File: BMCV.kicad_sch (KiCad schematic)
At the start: 32 parts, among them J13 DebugPins, J14 USB_C_Receptacle_USB2.0_14P, SW14 Reset, SW15 Boot, U32 TXS0108EPW, U36 STM32G474CETx, U37 MB85RS64PNF-G-JNERE1, Y1 38.4MHz 10pF

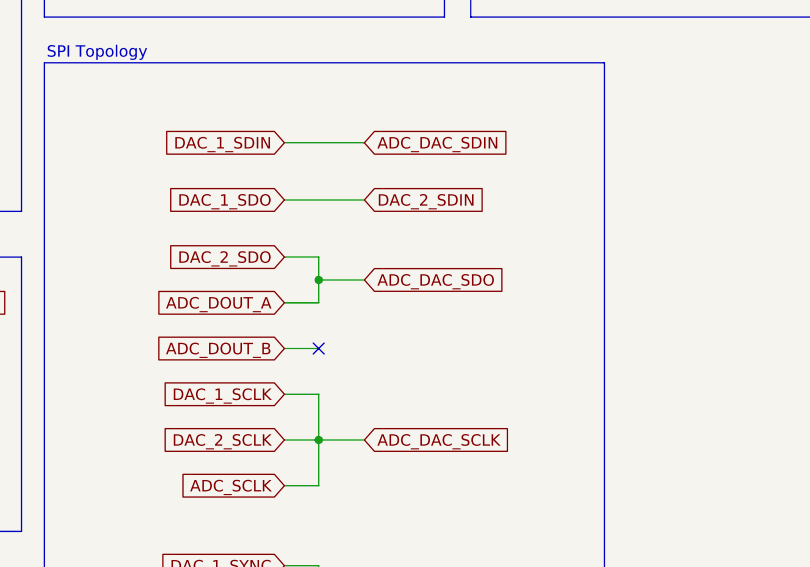
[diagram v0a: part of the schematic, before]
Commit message: pcb changes
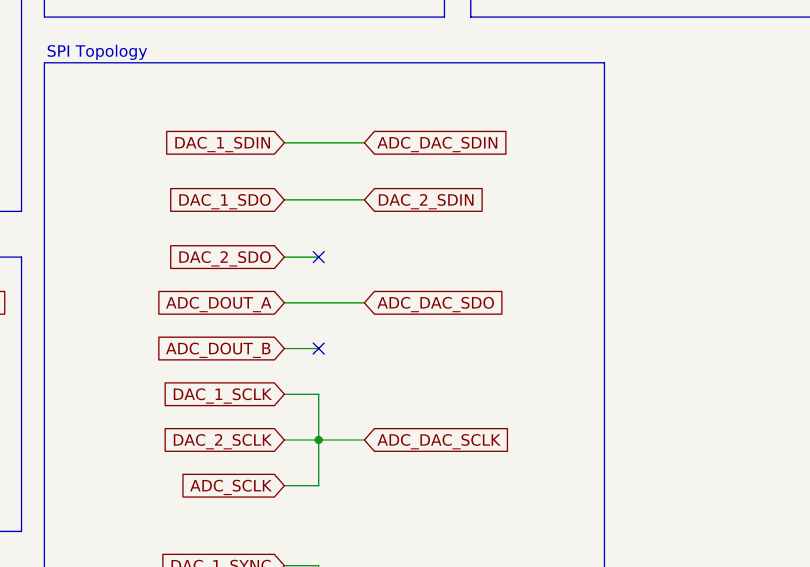
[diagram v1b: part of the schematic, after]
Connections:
- no-connect marks 3 -> 4
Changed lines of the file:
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@@
 	)
 	(junction
-		(at 140.97 175.26)
-		(diameter 0)
-		(color 0 0 0 0)
-	)
-	(junction
 		(at 29.21 237.49)
 		(diameter 0)
@@
 	)
 	(no_connect
+		(at 140.97 172.72)
+	)
+	(no_connect
 		(at 64.77 114.3)
 	)
@@
 	(wire
 		(pts
-			(xy 140.97 177.8) (xy 137.16 177.8)
+			(xy 137.16 177.8) (xy 146.05 177.8)
 		)
 		(stroke
@@
 	(wire
 		(pts
-			(xy 140.97 172.72) (xy 140.97 175.26)
-		)
-		(stroke
-			(width 0)
-			(type default)
-		)
-	)
-	(wire
-		(pts
 			(xy 118.11 269.24) (xy 128.27 269.24)
 		)
@@
 	(wire
 		(pts
-			(xy 140.97 175.26) (xy 146.05 175.26)
-		)
-		(stroke
-			(width 0)
-			(type default)
-		)
-	)
-	(wire
-		(pts
 			(xy 20.32 157.48) (xy 20.32 146.05)
 		)
@@
 	(wire
 		(pts
-			(xy 140.97 175.26) (xy 140.97 177.8)
-		)
-		(stroke
-			(width 0)
-			(type default)
-		)
-	)
-	(wire
-		(pts
 			(xy 69.85 257.81) (xy 72.39 257.81)
 		)
@@
 	(global_label "ADC_DAC_SDO"
 		(shape input)
-		(at 146.05 175.26 0)
+		(at 146.05 177.8 0)
 		(fields_autoplaced yes)
 		(effects
@@
 		)
 		(property "Intersheetrefs" "${INTERSHEET_REFS}"
-			(at 162.0376 175.26 0)
+			(at 162.0376 177.8 0)
 			(effects
 				(font

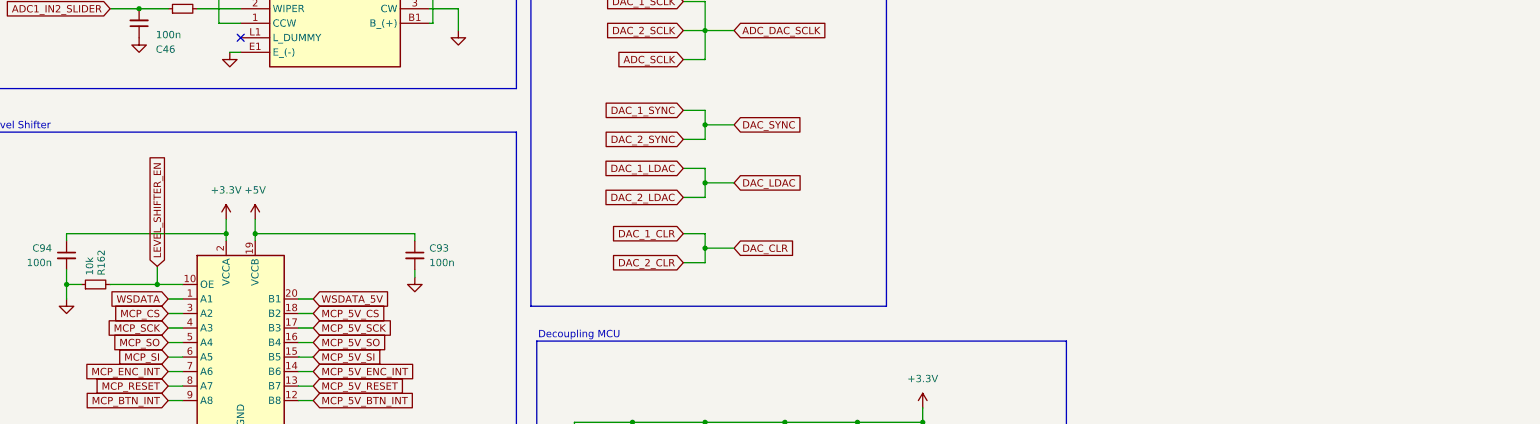
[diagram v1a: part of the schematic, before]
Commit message: pcb
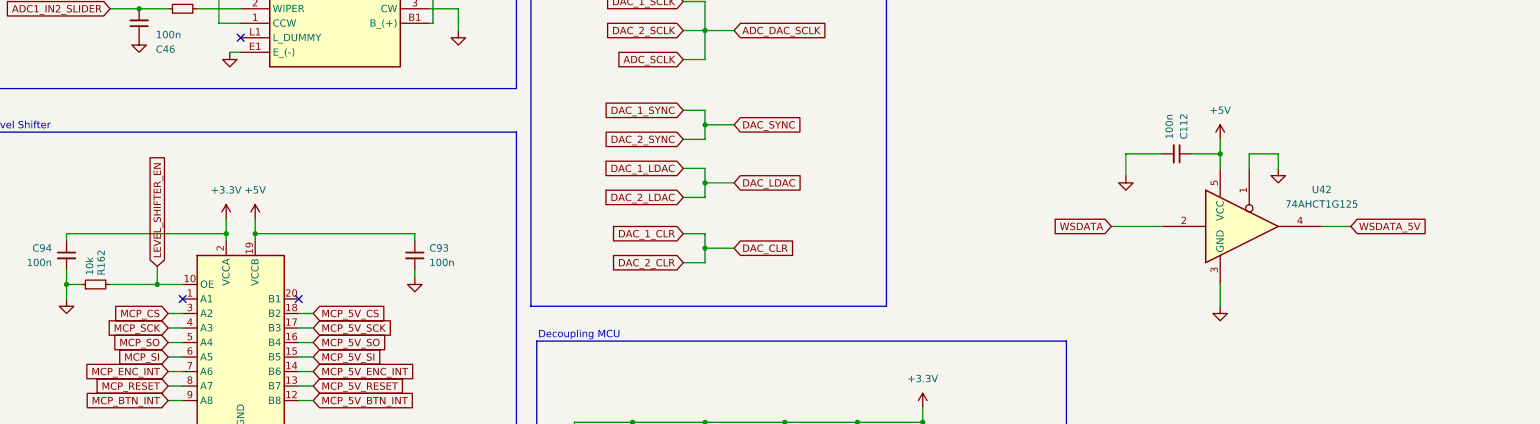
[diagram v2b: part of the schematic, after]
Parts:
- added C112: 100n, Capacitor_SMD:C_0402_1005Metric, symbol Device:C_Small
- added U42: 74AHCT1G125, Package_TO_SOT_SMD:SOT-353_SC-70-5, symbol 74xGxx:74AHCT1G125
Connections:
- net +5V: now also C112.1, U42.5 (VCC)
- net GND: now also C112.2, U42.1, U42.3 (GND)
- net WSDATA: now also U42.2; no longer U32.1 (A1)
- net WSDATA_5V: now also U42.4; no longer U32.20 (B1)
- no-connect marks 4 -> 6

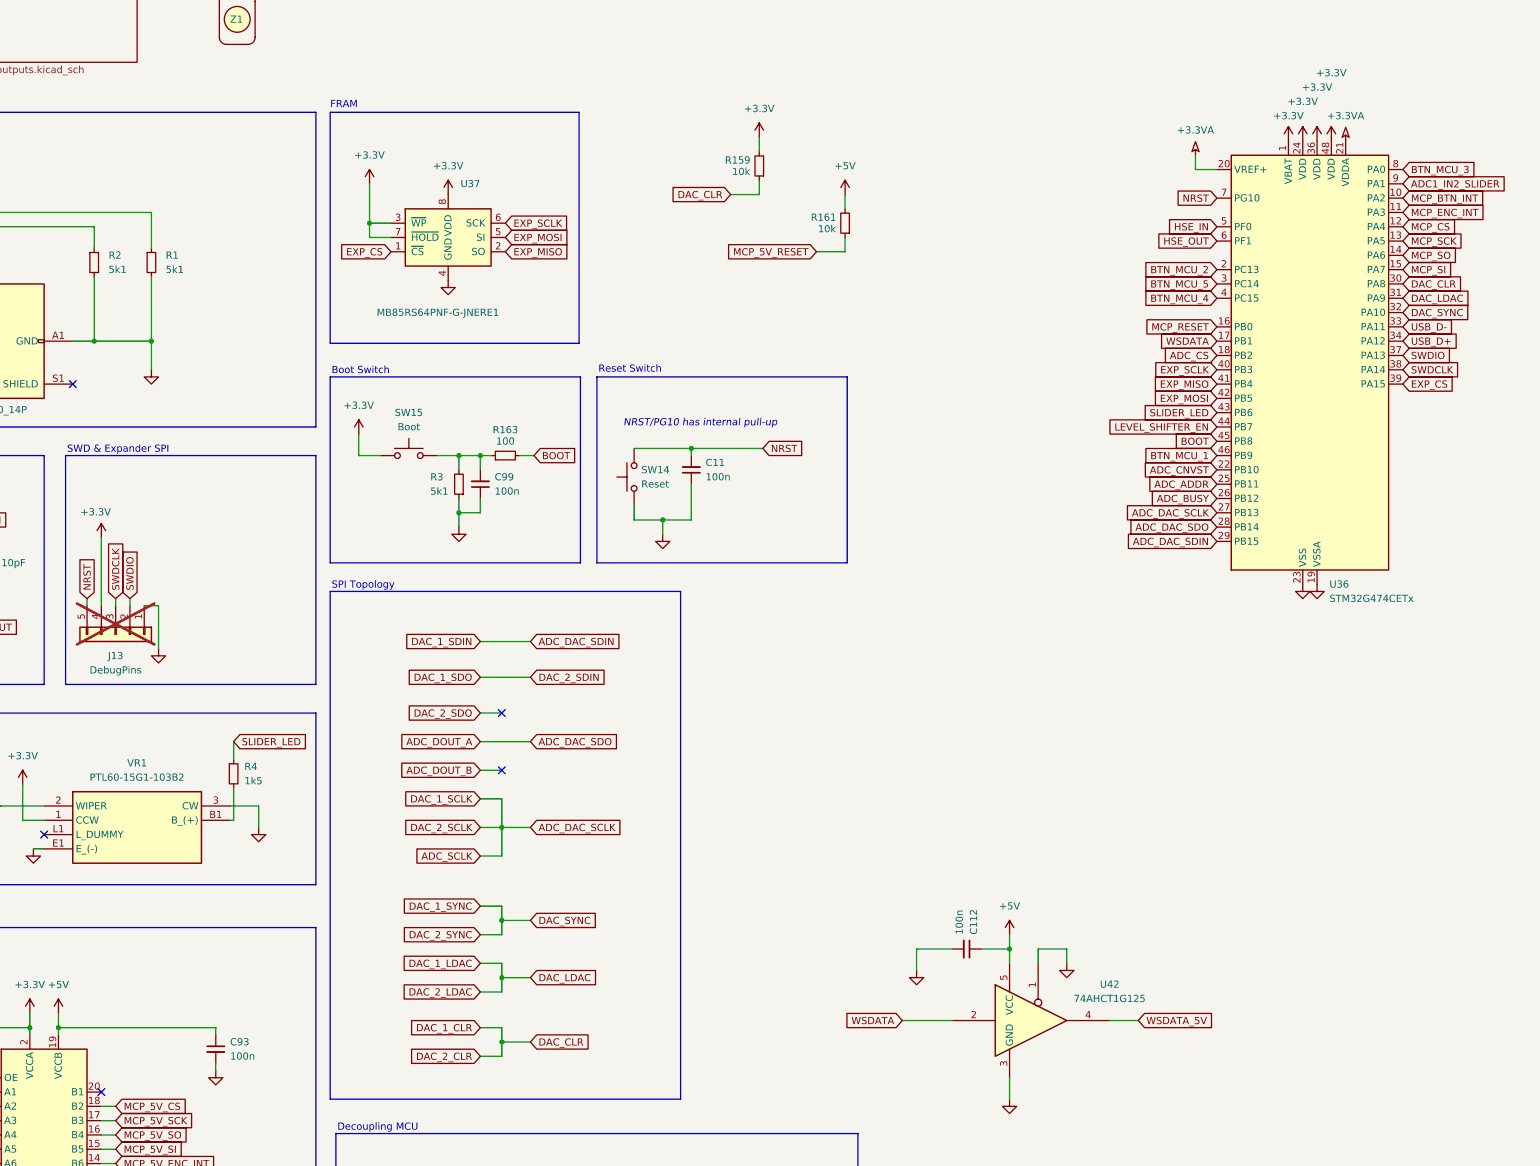
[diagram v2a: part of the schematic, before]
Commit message: pcb update
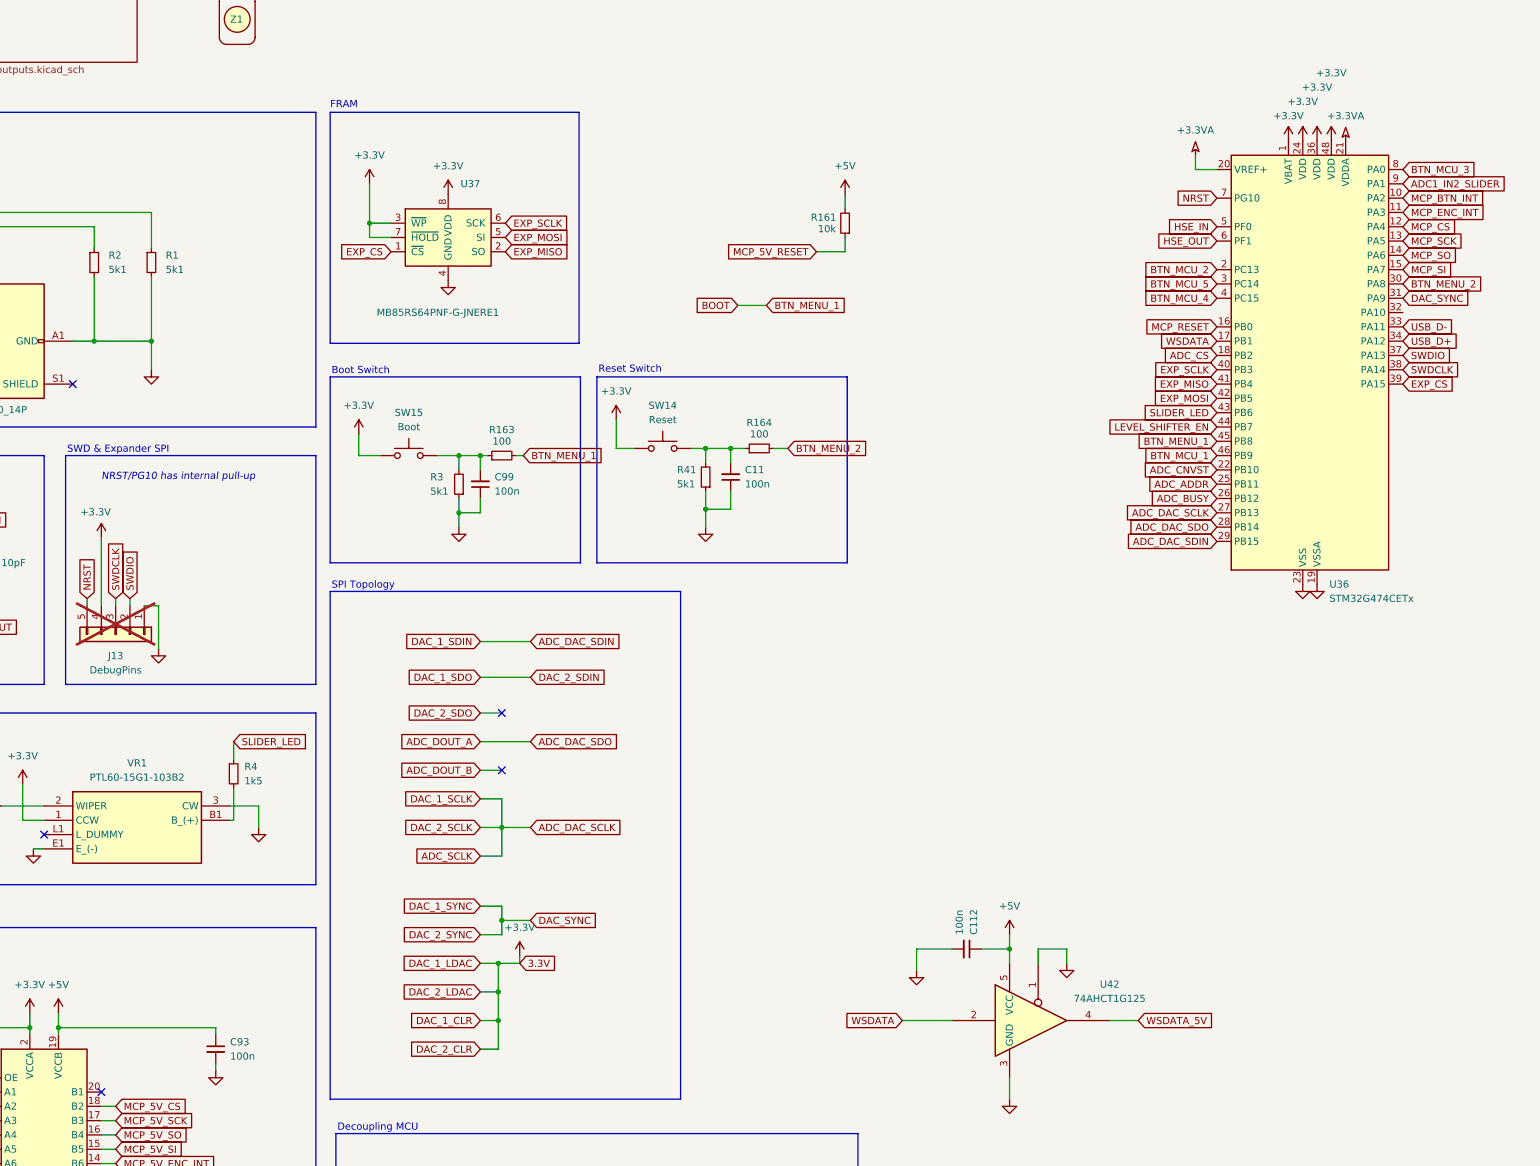
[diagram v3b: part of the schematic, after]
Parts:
- removed R159: 10k, Resistor_SMD:R_0402_1005Metric, symbol Device:R_Small
- added R164: 100, Resistor_SMD:R_0402_1005Metric, symbol Device:R_Small
- added R41: 5k1, Resistor_SMD:R_0402_1005Metric, symbol Device:R_Small
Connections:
- net DAC_1_LDAC is gone; now on net DAC_1_SYNC: U36.31 (PA9)
- net +3.3V: now also SW14.1
- net DAC_1_SYNC: no longer U36.32 (PA10)
- net GND: now also R41.1; no longer SW14.1
- net NRST: no longer C11.2, SW14.2
- net DAC_1_CLR renamed BTN_MENU_2
- net BTN_MENU_2: now also R164.2
- new net: C11.2, R164.1, R41.2, SW14.2
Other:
- moved on the sheet: C11, R163, SW14

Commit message: v1
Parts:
- removed C11, C99: 100n, Capacitor_SMD:C_0402_1005Metric, symbol Device:C_Small
- removed R4: 1k5, Resistor_SMD:R_0603_1608Metric, symbol Device:R_Small
- removed VR1: PTL60-15G1-103B2, BMCV:PTL6015xxxxxxx, symbol BMCV:PTLxx-xxxx-xxxxx
- added J13: EXTRA_PIN_1, TestPoint:TestPoint_Pad_D1.5mm, symbol Connector:Conn_01x01_Pin
- added R159, R160, R165, R166, R167, R169, R170: 10k, Resistor_SMD:R_0402_1005Metric, symbol Device:R_Small
- added R168: 100, Resistor_SMD:R_0402_1005Metric, symbol Device:R_Small
- added RV13: R_Potentiometer_Dual, BMCV:ALPHA_B10KX2, symbol Device:R_Potentiometer_Dual
- added SW16: FN3, BMCV:TS-1095PS-AXXBX-C3DX, symbol Switch:SW_Push
- R158: value 5k1 -> 1k; LCSC Part # C25905 -> C11702
- R3, R41: value 5k1 -> 10k; LCSC Part # C25905 -> C25744
- SW14: value Reset -> FN1
- SW15: value Boot -> FN2/Boot
- renumbered J13 to Jw1
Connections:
- net +3.3V: now also Jw1.2 (Pin_2), R165.1, R166.1, R169.1, R170.1, RV13.1, RV13.4, SW16.1; no longer Jw1.4 (Pin_4), U37.3 (~{WP}), U37.7 (~{HOLD})
- net DAC_1_SYNC: now also U36.32 (PA10); no longer U36.31 (PA9)
- net GND: now also R159.1, R160.1, R167.1, RV13.3, RV13.6
- net SWDCLK: now also Jw1.4 (Pin_4); no longer Jw1.3 (Pin_3)
- net SWDIO: now also Jw1.3 (Pin_3); no longer Jw1.2 (Pin_2)
- net at R158.2: now also RV13.5
- net SLIDER_LED renamed BTN_MENU_3
- net BTN_MENU_3: now also R168.2
- new net: R169.2, U37.7 (~{HOLD})
- new net: R170.2, U37.3 (~{WP})
- new net: R167.2, R168.1, SW16.2
- new net DAC_1_CLR: R165.2
- new net DAC_1_LDAC: R159.2
- new net DAC_2_CLR: R166.2
- new net DAC_2_LDAC: R160.2
- new net EXTRA_PIN_1: J13.1 (Pin_1), U36.31 (PA9)
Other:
- note added: "FN1/Boot Button"
- note added: "FN2 Button"
- note added: "FN3 Button"
- note removed: "Boot Switch"
- note removed: "Reset Switch"
- moved on the sheet: C46, R158, R163, R164, R3, R41, SW14, SW15
